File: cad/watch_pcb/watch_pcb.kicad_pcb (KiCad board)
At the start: 4 copper layers, 34 x 40 mm, 85 parts, among them J1 DISPLAY, J2 Micro_SD_Card, J4 USB_C_Receptacle, U1 LIS3MDL, U10 MX25LM51245GXDI00, U11 LSM6DSV16XTR, U2 MAX-M10M, U3 AMS1117-3.3, U5 AP131-18, U6 MAX30102, U7 MCP73871-2AA, U8 ESP32-S3, U9 S80KS5123GABHI020

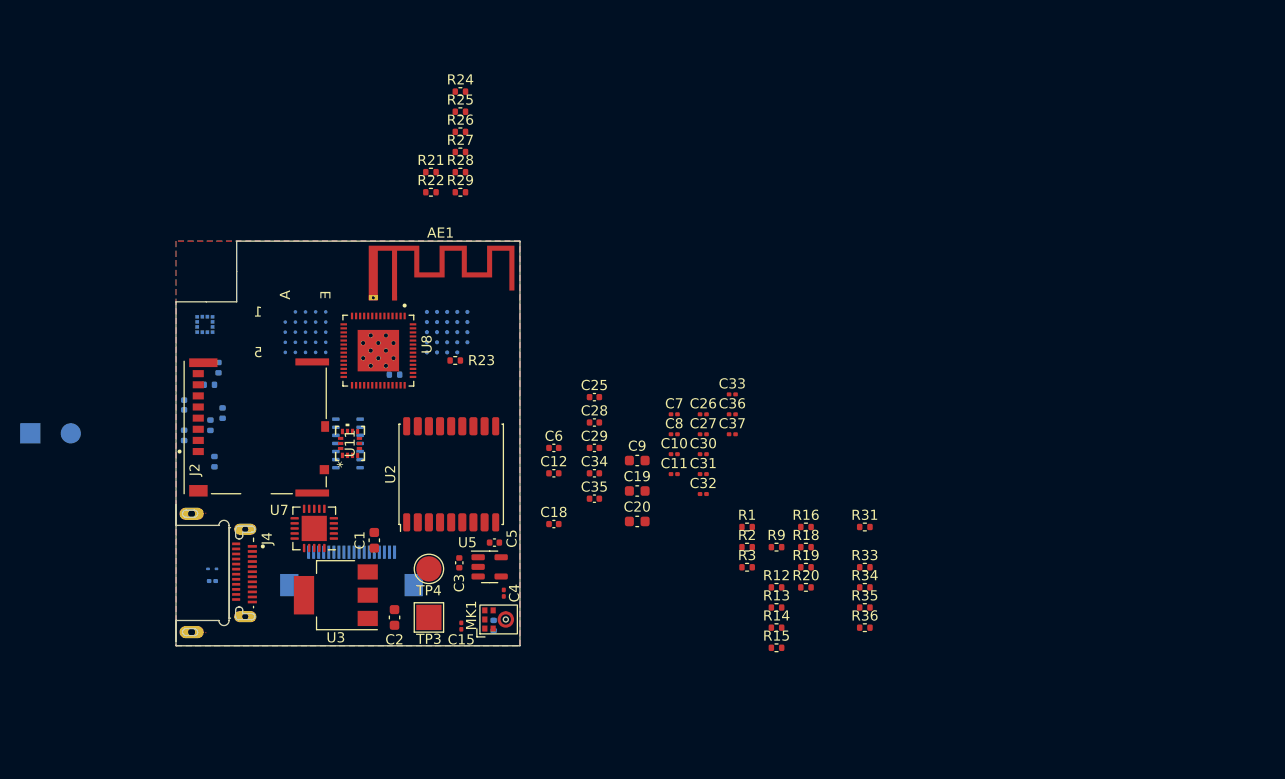
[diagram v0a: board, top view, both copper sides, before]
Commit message: idk some stuff
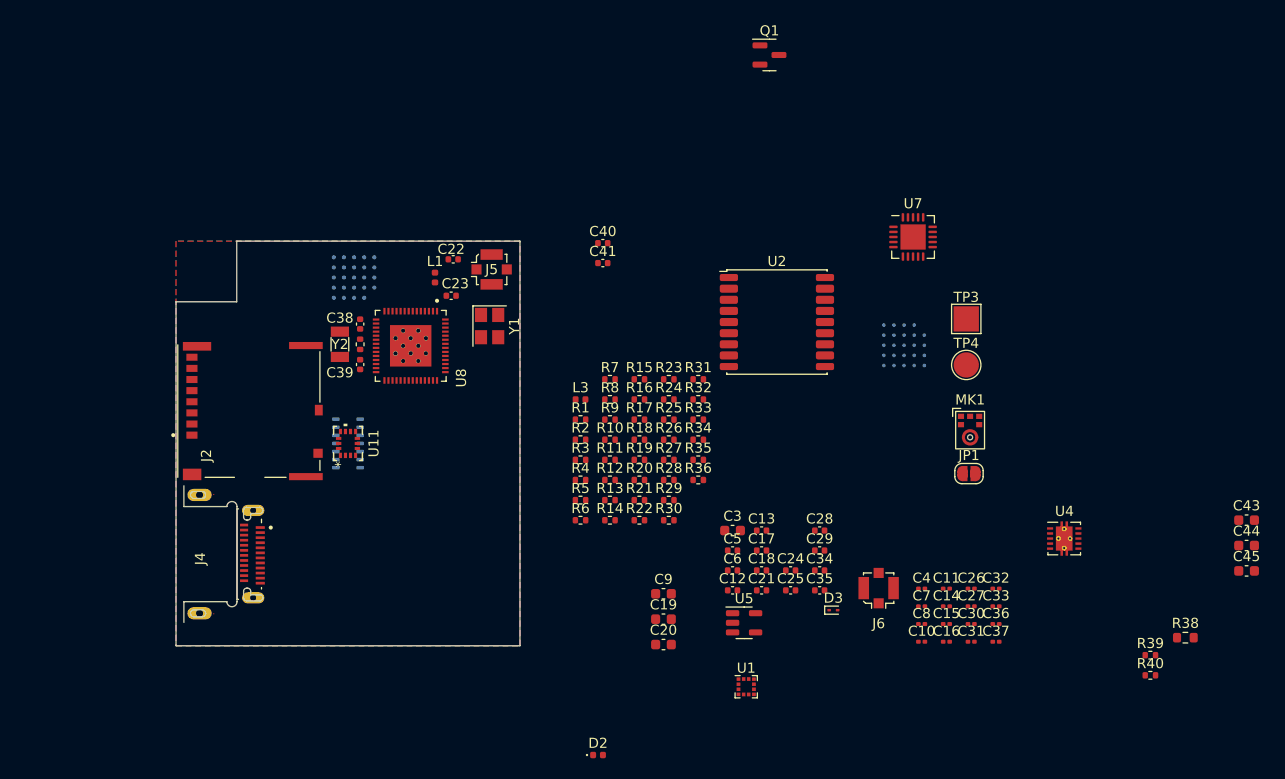
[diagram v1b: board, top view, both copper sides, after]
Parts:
- removed AE1: Antenna_Dipole, RF_Antenna:Texas_SWRA117D_2.4GHz_Right
- removed C1, C2: 22uF, Capacitor_SMD:C_0603_1608Metric
- removed J1: DISPLAY, Connector_FFC-FPC:Hirose_FH12-18S-0.5SH_1x18-1MP_P0.50mm_Horizontal
- removed TP1: BOOT, TestPoint:TestPoint_Pad_D2.0mm
- removed TP2: GND, TestPoint:TestPoint_Pad_2.0x2.0mm
- removed U3: AMS1117-3.3, Package_TO_SOT_SMD:SOT-223-3_TabPin2
- added C16: 100nF, Capacitor_SMD:C_0201_0603Metric, F.Cu at (176.6, 108.0)
- added C17: 1uF, Capacitor_SMD:C_0402_1005Metric, F.Cu at (158.3, 99.0)
- added C21: C, Capacitor_SMD:C_0402_1005Metric, F.Cu at (158.3, 102.9)
- added C22: 1.5pF, Capacitor_SMD:C_0402_1005Metric, F.Cu at (127.8, 70.2)
- added C23: 1.5pF, Capacitor_SMD:C_0402_1005Metric, F.Cu at (127.6, 73.8)
- added C24: C, Capacitor_SMD:C_0402_1005Metric, F.Cu at (161.2, 101.0)
- added C38: C, Capacitor_SMD:C_0402_1005Metric, F.Cu at (118.6, 76.6)
- added C39: C, Capacitor_SMD:C_0402_1005Metric, F.Cu at (118.6, 80.6)
- added C40: C, Capacitor_SMD:C_0402_1005Metric, F.Cu at (142.6, 68.6)
- added C41: C, Capacitor_SMD:C_0402_1005Metric, F.Cu at (142.6, 70.6)
- added C43: 10uF, Capacitor_SMD:C_0603_1608Metric, F.Cu at (206.2, 96.0)
- added C44: 10uF, Capacitor_SMD:C_0603_1608Metric, F.Cu at (206.2, 98.5)
- added C45: 10uF, Capacitor_SMD:C_0603_1608Metric, F.Cu at (206.2, 101.0)
- added D2: CHG_STATUS, LED_SMD:LED_0402_1005Metric, F.Cu at (142.1, 119.2)
- added J5: ESP_ANT, Connector_Coaxial:U.FL_Molex_MCRF_73412-0110_Vertical, F.Cu at (131.6, 71.2)
- added J6: GPS_ANT, Connector_Coaxial:U.FL_Molex_MCRF_73412-0110_Vertical, F.Cu at (169.9, 102.7)
- added JP1: BOOT, Jumper:SolderJumper-2_P1.3mm_Open_RoundedPad1.0x1.5mm, F.Cu at (178.8, 91.4)
- added L1: 2.7nH, Inductor_SMD:L_0402_1005Metric, F.Cu at (126.0, 72.0)
- added L3: 2nH, Inductor_SMD:L_0402_1005Metric, F.Cu at (140.4, 84.0)
- added Q1: BC818, Package_TO_SOT_SMD:SOT-23, F.Cu at (159.1, 50.0)
- added R10: 10k, Resistor_SMD:R_0402_1005Metric, F.Cu at (143.3, 88.0)
- added R17: 0, Resistor_SMD:R_0402_1005Metric, F.Cu at (146.2, 86.0)
- added R37: R, Resistor_SMD:R_0402_1005Metric, F.Cu at (118.6, 78.6)
- added R38: 10, Resistor_SMD:R_0603_1608Metric, F.Cu at (200.2, 107.6)
- added R39: 1k, Resistor_SMD:R_0402_1005Metric, F.Cu at (196.7, 109.3)
- added R40: 100, Resistor_SMD:R_0402_1005Metric, F.Cu at (196.7, 111.3)
- added U4: TPS63001, Package_SON:Texas_DRC0010J_ThermalVias, F.Cu at (188.2, 97.8)
- added Y1: 40MHz(10ppm), Crystal:Crystal_SMD_3225-4Pin_3.2x2.5mm, F.Cu at (131.4, 76.8)
- added Y2: 32.768kHz, Crystal:Crystal_SMD_3215-2Pin_3.2x1.5mm, F.Cu at (116.6, 78.6)
- C13, C14, D3, R11, R30, R32, R4, R5, R6, R7, R8, U1: moved to F.Cu
- C3: footprint Capacitor_SMD:C_0402_1005Metric -> Capacitor_SMD:C_0603_1608Metric
- TP3: value BATT- -> Conn_B-
- TP4: value BATT+ -> Conn_B+
- U2: value MAX-M10M -> MAX-M10S
- moved C14 72.6 mm to (176.6, 104.5), turned to 0 degrees
- moved U7 65.8 mm to (173.3, 68.0), turned to 0 degrees
- moved U1 64.4 mm to (156.8, 112.5), turned to 0 degrees
- moved D3 61.5 mm to (165.4, 104.9), turned to 0 degrees
- moved TP3 60.8 mm to (178.5, 76.1), turned to 0 degrees
- moved U10 59.2 mm to (172.4, 78.7), turned to 180 degrees
- moved C13 58.4 mm to (158.3, 97.0), turned to 0 degrees
- moved TP4 56.8 mm to (178.5, 80.6), turned to 0 degrees
- moved MK1 50.2 mm to (178.9, 87.1), turned to 0 degrees
- moved R32 48.2 mm to (152.0, 84.0), turned to 0 degrees
- moved C15 48.0 mm to (176.6, 106.2), turned to 0 degrees
- moved R8 42.2 mm to (143.3, 84.0), turned to 0 degrees
- moved C4 41.3 mm to (174.1, 102.8), turned to 0 degrees
- moved R7 39.8 mm to (143.3, 82.1), turned to 0 degrees
- moved R6 38.8 mm to (140.4, 96.0), turned to 0 degrees
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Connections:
- net /GPIO47 renamed /BTN1
- net /GPIO48 renamed /BTN2
- net /SPI2_CS0 renamed /DISP_CS
- net Net-(U8-GPIO46) renamed /DISP_RESET
- R31 pad 1: /GPIO_45 -> /GPS_INT
- R33 pad 1: /I2C1_SCL -> /I2C0_SCL
- R34 pad 1: /I2C1_SDA -> /I2C0_SDA
- U11 pad 13: /I2C1_SCL -> /I2C0_SCL
- U11 pad 14: /I2C1_SDA -> /I2C0_SDA
- U2 pad 11: unconnected-(U2-RF_IN-Pad11) -> Net-(U2-RF_IN)
- U2 pad 16: unconnected-(U2-SDA-Pad16) -> /I2C1_SDA
- U2 pad 17: unconnected-(U2-SCL-Pad17) -> /I2C1_SCL
- U2 pad 5: unconnected-(U2-EXTINT-Pad5) -> /GPS_INT
- U7 pad 17: +1V8 -> +5V
- U7 pad 4: +1V8 -> +5V
- U8 pad 1: Net-(U8-LNA_IN) -> /ESP_ANT
- U8 pad 10: unconnected-(U8-GPIO5-Pad10) -> /BAT_STAT2
- U8 pad 11: unconnected-(U8-GPIO6-Pad11) -> /MIC_WS
- U8 pad 12: unconnected-(U8-GPIO7-Pad12) -> /MIC_SCK
- U8 pad 13: unconnected-(U8-GPIO8-Pad13) -> /MIC_SD
- U8 pad 14: /SPI2_ -> /BL_CTRL
- U8 pad 16: /SPI2_ -> /DISP_MOSI
- U8 pad 17: /SPI2_ -> /DISP_CLK
- U8 pad 18: /SPI2_ -> /DISP_DC
- U8 pad 19: /SPI2_ -> /TP_INT
- U8 pad 21: unconnected-(U8-XTAL_32K_P-Pad21) -> /RTC_P
- U8 pad 22: unconnected-(U8-XTAL_32K_N-Pad22) -> /RTC_N
- U8 pad 23: unconnected-(U8-GPIO17-Pad23) -> /HBT_INT
- U8 pad 24: unconnected-(U8-GPIO18-Pad24) -> /IMU_INT2
- U8 pad 25: unconnected-(U8-GPIO19-Pad25) -> /USB_DM
- U8 pad 26: unconnected-(U8-GPIO20-Pad26) -> /USB_DM
- U8 pad 27: unconnected-(U8-GPIO21-Pad27) -> /IMU_Wakeup
- U8 pad 43: unconnected-(U8-GPIO38-Pad43) -> /LED_EN
- U8 pad 44: /GPIO39 -> /SD_D0
- U8 pad 45: /GPIO40 -> /SD_D1
- U8 pad 47: /GPIO41 -> /SD_D2
- U8 pad 48: /GPIO42 -> /SD_D3
- U8 pad 49: unconnected-(U8-U0TXD-Pad49) -> /SD_CLK
- U8 pad 5: /I2C1_SCL -> /I2C0_SCL
- U8 pad 50: unconnected-(U8-U0RXD-Pad50) -> /SD_CMD
- U8 pad 51: /GPIO_45 -> /GPS_INT
- U8 pad 53: unconnected-(U8-XTAL_N-Pad53) -> /CLK_N
- U8 pad 54: unconnected-(U8-XTAL_P-Pad54) -> /CLK_P
- U8 pad 6: /I2C1_SDA -> /I2C0_SDA
- U8 pad 7: unconnected-(U8-GPIO2-Pad7) -> /I2C1_SCL
- U8 pad 8: unconnected-(U8-GPIO3-Pad8) -> /I2C1_SDA
- U8 pad 9: unconnected-(U8-GPIO4-Pad9) -> /BAT_STAT1
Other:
- outline, holes or cut-outs redrawn
